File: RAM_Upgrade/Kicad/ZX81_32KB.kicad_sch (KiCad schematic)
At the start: 3 parts, among them IC1 CY62256NLL-55SNXI, J3 Conn_01x04_Pin, J4 828-AG11D-LF

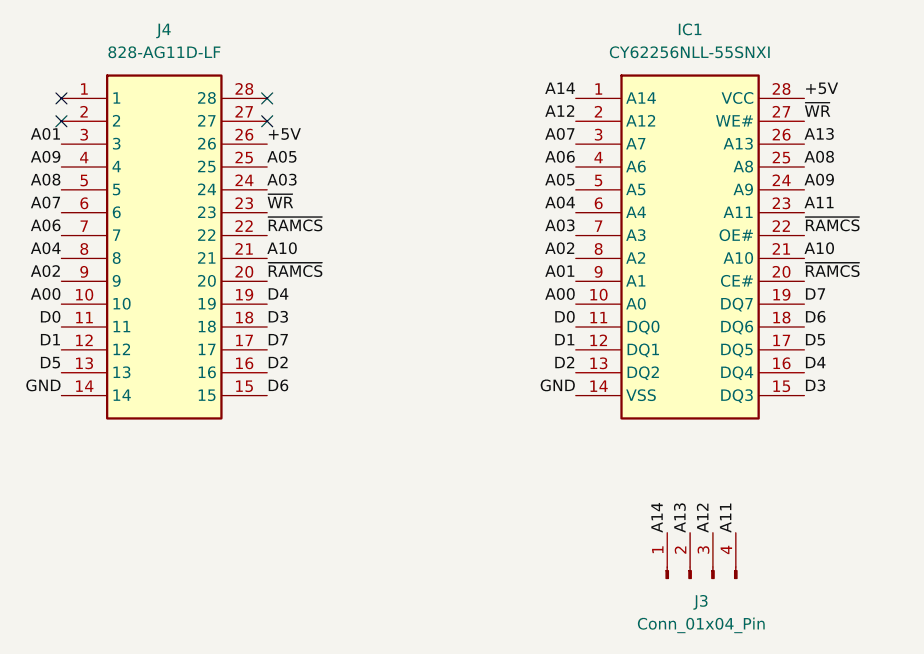
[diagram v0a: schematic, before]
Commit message: Corrected initial version
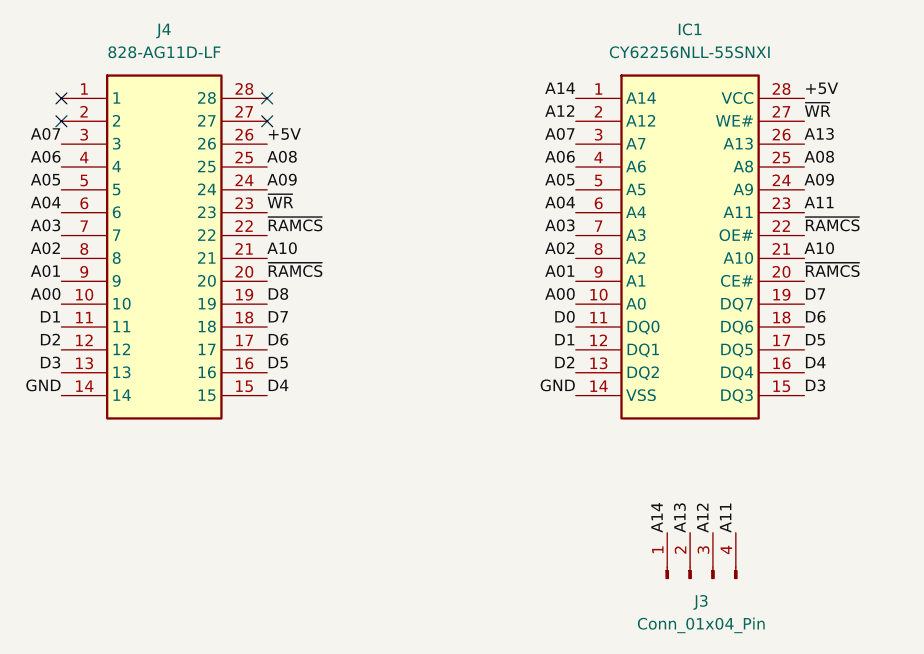
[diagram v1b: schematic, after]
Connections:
- net A01: now also J4.9; no longer J4.3
- net A02: now also J4.8; no longer J4.9
- net A03: now also J4.7; no longer J4.24
- net A04: now also J4.6; no longer J4.8
- net A05: now also J4.5; no longer J4.25
- net A06: now also J4.4; no longer J4.7
- net A07: now also J4.3; no longer J4.6
- net A08: now also J4.25; no longer J4.5
- net A09: now also J4.24; no longer J4.4
- net D0: no longer J4.11
- net D1: now also J4.11; no longer J4.12
- net D2: now also J4.12; no longer J4.16
- net D3: now also J4.13; no longer J4.18
- net D4: now also J4.15; no longer J4.19
- net D5: now also J4.16; no longer J4.13
- net D6: now also J4.17; no longer J4.15
- net D7: now also J4.18; no longer J4.17
- new net D8: J4.19
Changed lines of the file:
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@@
   (no_connect (at 52.07 64.77))
   (no_connect (at 74.93 64.77))
-  (label "A01" (at 52.07 67.31 180) (fields_autoplaced)
+  (label "A07" (at 52.07 67.31 180) (fields_autoplaced)
     (effects (font (size 1.27 1.27)) (justify right bottom))
   )
-  (label "A02" (at 52.07 82.55 180) (fields_autoplaced)
+  (label "A01" (at 52.07 82.55 180) (fields_autoplaced)
     (effects (font (size 1.27 1.27)) (justify right bottom))
   )
@@
     (effects (font (size 1.27 1.27)) (justify left bottom))
   )
-  (label "D2" (at 74.93 92.71 0) (fields_autoplaced)
+  (label "D5" (at 74.93 92.71 0) (fields_autoplaced)
     (effects (font (size 1.27 1.27)) (justify left bottom))
   )
@@
     (effects (font (size 1.27 1.27)) (justify right bottom))
   )
-  (label "D7" (at 74.93 90.17 0) (fields_autoplaced)
+  (label "D6" (at 74.93 90.17 0) (fields_autoplaced)
     (effects (font (size 1.27 1.27)) (justify left bottom))
   )
@@
     (effects (font (size 1.27 1.27)) (justify right bottom))
   )
-  (label "D3" (at 74.93 87.63 0) (fields_autoplaced)
+  (label "D7" (at 74.93 87.63 0) (fields_autoplaced)
     (effects (font (size 1.27 1.27)) (justify left bottom))
   )
@@
     (effects (font (size 1.27 1.27)) (justify right bottom))
   )
-  (label "D5" (at 52.07 92.71 180) (fields_autoplaced)
+  (label "D3" (at 52.07 92.71 180) (fields_autoplaced)
     (effects (font (size 1.27 1.27)) (justify right bottom))
   )
-  (label "A06" (at 52.07 77.47 180) (fields_autoplaced)
+  (label "A03" (at 52.07 77.47 180) (fields_autoplaced)
     (effects (font (size 1.27 1.27)) (justify right bottom))
   )
@@
     (effects (font (size 1.27 1.27)) (justify left bottom))
   )
-  (label "D6" (at 74.93 95.25 0) (fields_autoplaced)
+  (label "D4" (at 74.93 95.25 0) (fields_autoplaced)
     (effects (font (size 1.27 1.27)) (justify left bottom))
   )
@@
     (effects (font (size 1.27 1.27)) (justify right bottom))
   )
-  (label "A05" (at 74.93 69.85 0) (fields_autoplaced)
+  (label "A08" (at 74.93 69.85 0) (fields_autoplaced)
     (effects (font (size 1.27 1.27)) (justify left bottom))
   )
-  (label "A04" (at 52.07 80.01 180) (fields_autoplaced)
+  (label "A02" (at 52.07 80.01 180) (fields_autoplaced)
     (effects (font (size 1.27 1.27)) (justify right bottom))
   )
@@
     (effects (font (size 1.27 1.27)) (justify left bottom))
   )
-  (label "D4" (at 74.93 85.09 0) (fields_autoplaced)
+  (label "D8" (at 74.93 85.09 0) (fields_autoplaced)
     (effects (font (size 1.27 1.27)) (justify left bottom))
   )
@@
     (effects (font (size 1.27 1.27)) (justify left bottom))
   )
-  (label "A03" (at 74.93 72.39 0) (fields_autoplaced)
+  (label "A09" (at 74.93 72.39 0) (fields_autoplaced)
     (effects (font (size 1.27 1.27)) (justify left bottom))
   )
@@
     (effects (font (size 1.27 1.27)) (justify left bottom))
   )
-  (label "D0" (at 52.07 87.63 180) (fields_autoplaced)
+  (label "D1" (at 52.07 87.63 180) (fields_autoplaced)
     (effects (font (size 1.27 1.27)) (justify right bottom))
   )
@@
     (effects (font (size 1.27 1.27)) (justify right bottom))
   )
-  (label "A08" (at 52.07 72.39 180) (fields_autoplaced)
+  (label "A05" (at 52.07 72.39 180) (fields_autoplaced)
     (effects (font (size 1.27 1.27)) (justify right bottom))
   )
@@
     (effects (font (size 1.27 1.27)) (justify left bottom))
   )
-  (label "A07" (at 52.07 74.93 180) (fields_autoplaced)
+  (label "A04" (at 52.07 74.93 180) (fields_autoplaced)
     (effects (font (size 1.27 1.27)) (justify right bottom))
   )
@@
     (effects (font (size 1.27 1.27)) (justify left bottom))
   )
-  (label "D1" (at 52.07 90.17 180) (fields_autoplaced)
+  (label "D2" (at 52.07 90.17 180) (fields_autoplaced)
     (effects (font (size 1.27 1.27)) (justify right bottom))
   )
@@
     (effects (font (size 1.27 1.27)) (justify left bottom))
   )
-  (label "A09" (at 52.07 69.85 180) (fields_autoplaced)
+  (label "A06" (at 52.07 69.85 180) (fields_autoplaced)
     (effects (font (size 1.27 1.27)) (justify right bottom))
   )

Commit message: Revert to original design
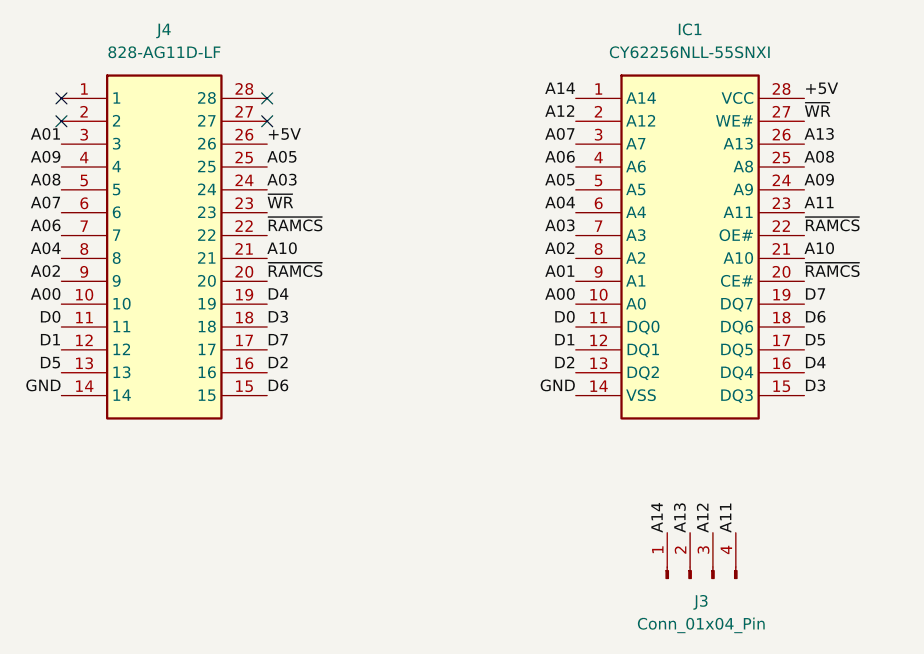
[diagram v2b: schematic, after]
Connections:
- net D8 is gone; now on net D4: J4.19
- net A01: now also J4.3; no longer J4.9
- net A02: now also J4.9; no longer J4.8
- net A03: now also J4.24; no longer J4.7
- net A04: now also J4.8; no longer J4.6
- net A05: now also J4.25; no longer J4.5
- net A06: now also J4.7; no longer J4.4
- net A07: now also J4.6; no longer J4.3
- net A08: now also J4.5; no longer J4.25
- net A09: now also J4.4; no longer J4.24
- net D0: now also J4.11
- net D1: now also J4.12; no longer J4.11
- net D2: now also J4.16; no longer J4.12
- net D3: now also J4.18; no longer J4.13
- net D4: no longer J4.15
- net D5: now also J4.13; no longer J4.16
- net D6: now also J4.15; no longer J4.17
- net D7: now also J4.17; no longer J4.18
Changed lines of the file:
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@@
   (no_connect (at 52.07 64.77))
   (no_connect (at 74.93 64.77))
-  (label "A07" (at 52.07 67.31 180) (fields_autoplaced)
+  (label "A01" (at 52.07 67.31 180) (fields_autoplaced)
     (effects (font (size 1.27 1.27)) (justify right bottom))
   )
-  (label "A01" (at 52.07 82.55 180) (fields_autoplaced)
+  (label "A02" (at 52.07 82.55 180) (fields_autoplaced)
     (effects (font (size 1.27 1.27)) (justify right bottom))
   )
@@
     (effects (font (size 1.27 1.27)) (justify left bottom))
   )
-  (label "D5" (at 74.93 92.71 0) (fields_autoplaced)
+  (label "D2" (at 74.93 92.71 0) (fields_autoplaced)
     (effects (font (size 1.27 1.27)) (justify left bottom))
   )
@@
     (effects (font (size 1.27 1.27)) (justify right bottom))
   )
-  (label "D6" (at 74.93 90.17 0) (fields_autoplaced)
+  (label "D7" (at 74.93 90.17 0) (fields_autoplaced)
     (effects (font (size 1.27 1.27)) (justify left bottom))
   )
@@
     (effects (font (size 1.27 1.27)) (justify right bottom))
   )
-  (label "D7" (at 74.93 87.63 0) (fields_autoplaced)
+  (label "D3" (at 74.93 87.63 0) (fields_autoplaced)
     (effects (font (size 1.27 1.27)) (justify left bottom))
   )
@@
     (effects (font (size 1.27 1.27)) (justify right bottom))
   )
-  (label "D3" (at 52.07 92.71 180) (fields_autoplaced)
+  (label "D5" (at 52.07 92.71 180) (fields_autoplaced)
     (effects (font (size 1.27 1.27)) (justify right bottom))
   )
-  (label "A03" (at 52.07 77.47 180) (fields_autoplaced)
+  (label "A06" (at 52.07 77.47 180) (fields_autoplaced)
     (effects (font (size 1.27 1.27)) (justify right bottom))
   )
@@
     (effects (font (size 1.27 1.27)) (justify left bottom))
   )
-  (label "D4" (at 74.93 95.25 0) (fields_autoplaced)
+  (label "D6" (at 74.93 95.25 0) (fields_autoplaced)
     (effects (font (size 1.27 1.27)) (justify left bottom))
   )
@@
     (effects (font (size 1.27 1.27)) (justify right bottom))
   )
-  (label "A08" (at 74.93 69.85 0) (fields_autoplaced)
+  (label "A05" (at 74.93 69.85 0) (fields_autoplaced)
     (effects (font (size 1.27 1.27)) (justify left bottom))
   )
-  (label "A02" (at 52.07 80.01 180) (fields_autoplaced)
+  (label "A04" (at 52.07 80.01 180) (fields_autoplaced)
     (effects (font (size 1.27 1.27)) (justify right bottom))
   )
@@
     (effects (font (size 1.27 1.27)) (justify left bottom))
   )
-  (label "D8" (at 74.93 85.09 0) (fields_autoplaced)
+  (label "D4" (at 74.93 85.09 0) (fields_autoplaced)
     (effects (font (size 1.27 1.27)) (justify left bottom))
   )
@@
     (effects (font (size 1.27 1.27)) (justify left bottom))
   )
-  (label "A09" (at 74.93 72.39 0) (fields_autoplaced)
+  (label "A03" (at 74.93 72.39 0) (fields_autoplaced)
     (effects (font (size 1.27 1.27)) (justify left bottom))
   )
@@
     (effects (font (size 1.27 1.27)) (justify left bottom))
   )
-  (label "D1" (at 52.07 87.63 180) (fields_autoplaced)
+  (label "D0" (at 52.07 87.63 180) (fields_autoplaced)
     (effects (font (size 1.27 1.27)) (justify right bottom))
   )
@@
     (effects (font (size 1.27 1.27)) (justify right bottom))
   )
-  (label "A05" (at 52.07 72.39 180) (fields_autoplaced)
+  (label "A08" (at 52.07 72.39 180) (fields_autoplaced)
     (effects (font (size 1.27 1.27)) (justify right bottom))
   )
@@
     (effects (font (size 1.27 1.27)) (justify left bottom))
   )
-  (label "A04" (at 52.07 74.93 180) (fields_autoplaced)
+  (label "A07" (at 52.07 74.93 180) (fields_autoplaced)
     (effects (font (size 1.27 1.27)) (justify right bottom))
   )
@@
     (effects (font (size 1.27 1.27)) (justify left bottom))
   )
-  (label "D2" (at 52.07 90.17 180) (fields_autoplaced)
+  (label "D1" (at 52.07 90.17 180) (fields_autoplaced)
     (effects (font (size 1.27 1.27)) (justify right bottom))
   )
@@
     (effects (font (size 1.27 1.27)) (justify left bottom))
   )
-  (label "A06" (at 52.07 69.85 180) (fields_autoplaced)
+  (label "A09" (at 52.07 69.85 180) (fields_autoplaced)
     (effects (font (size 1.27 1.27)) (justify right bottom))
   )
